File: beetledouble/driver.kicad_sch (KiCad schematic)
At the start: 15 parts, among them J5 motor_out, Q3 AON6884, Q4 AON6884, U6 ADP3110A, U7 ADP3110A

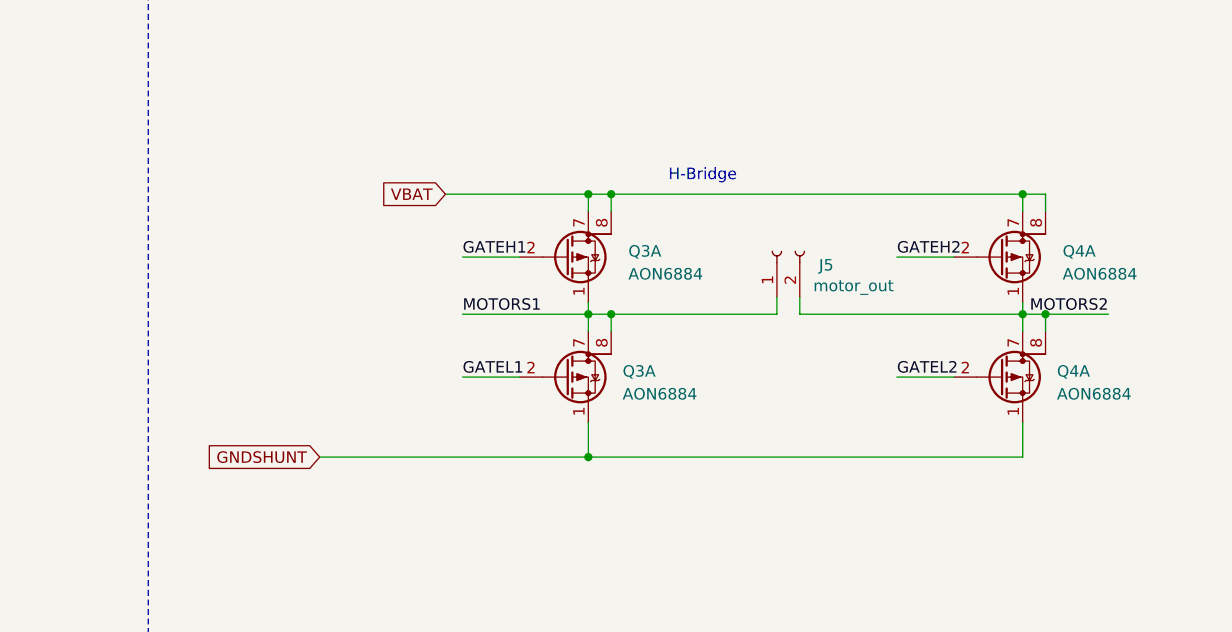
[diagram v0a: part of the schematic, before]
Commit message: Beetledouble ESC
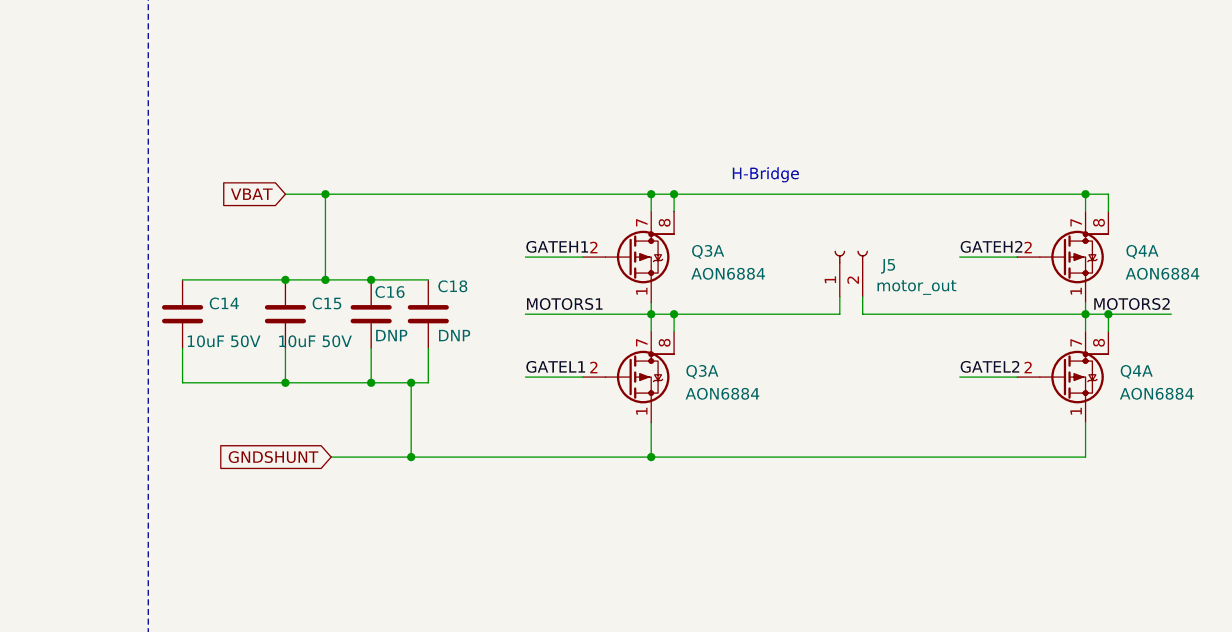
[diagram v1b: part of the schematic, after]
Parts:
- added C14, C15: 10uF 50V, Capacitor_SMD:C_1206_3216Metric, symbol Device:C
- added C16, C18: DNP, Capacitor_SMD:C_1206_3216Metric, symbol Device:C
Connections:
- net GNDSHUNT: now also C14.2, C15.2, C16.2, C18.2
- net VBAT: now also C14.1, C15.1, C16.1, C18.1
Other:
- moved on the sheet: J5, Q3A, Q4A
